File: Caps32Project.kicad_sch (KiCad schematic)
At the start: 35 parts, among them J1 PH2.0, J2 USB_C_Receptacle_USB2.0_16P, J3 SH1.0, Q1 AO3401A, SW1 Boot, SW2 Reset, SW3 SW_SPDT_312, U1 TP4057, U2 MPU-6050, U3 ESP32-C3-MINI-1, U4 AP2112K-3.3

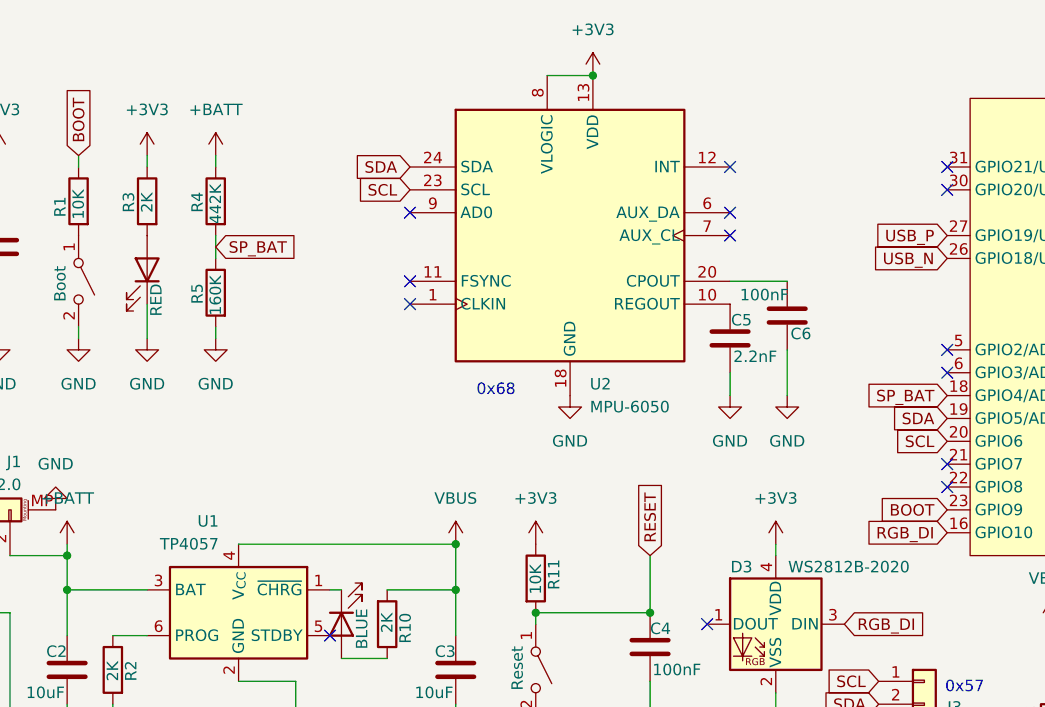
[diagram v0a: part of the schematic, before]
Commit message: Update Board
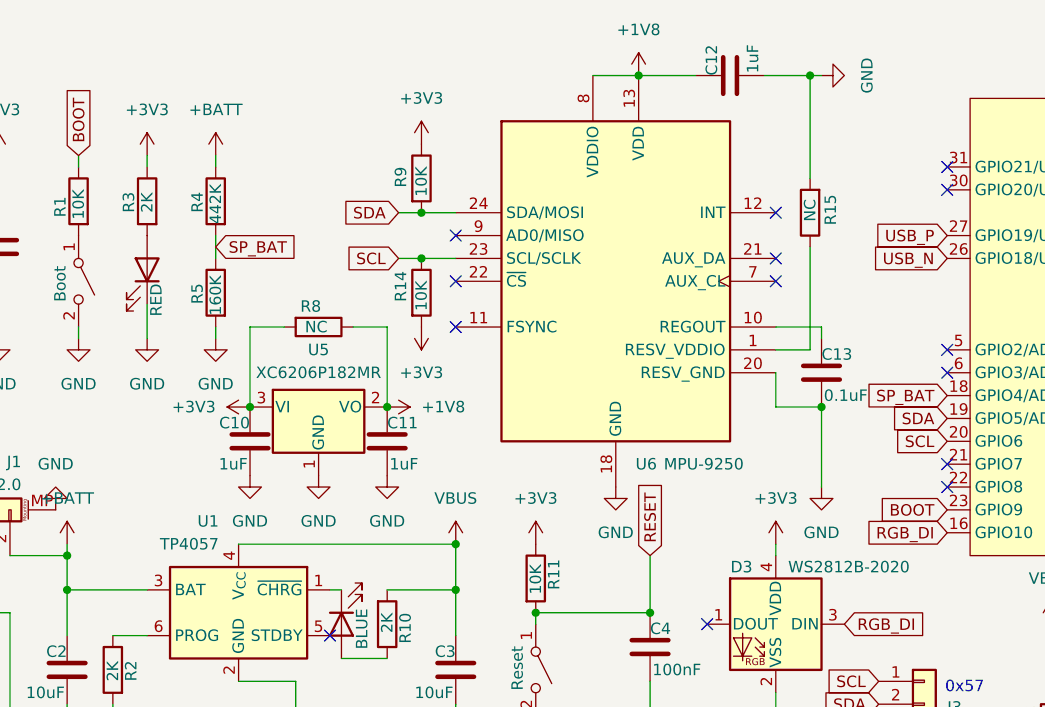
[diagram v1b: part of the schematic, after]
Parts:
- removed C5: 2.2nF, Capacitor_SMD:C_0603_1608Metric, symbol Device:C
- removed C6: 100nF, Capacitor_SMD:C_0402_1005Metric, symbol Device:C
- removed U2: MPU-6050, Sensor_Motion:InvenSense_QFN-24_4x4mm_P0.5mm, symbol Sensor_Motion:MPU-6050
- added C10, C11, C12: 1uF, Capacitor_SMD:C_0402_1005Metric, symbol Device:C
- added C13: 0.1uF, Capacitor_SMD:C_0402_1005Metric, symbol Device:C
- added R14, R9: 10K, Resistor_SMD:R_0402_1005Metric, symbol Device:R
- added R15, R8: NC, Resistor_SMD:R_0402_1005Metric, symbol Device:R
- added U5: XC6206P182MR, Package_TO_SOT_SMD:SOT-23-3, symbol Regulator_Linear:XC6206PxxxMR
- added U6: MPU-9250, Sensor_Motion:InvenSense_QFN-24_3x3mm_P0.4mm, symbol Sensor_Motion:MPU-9250
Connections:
- net +3V3: now also C10.1, R14.2, R8.2, R9.1, U5.3 (VI)
- net GND: now also C10.2, C11.2, C12.2, C13.2, R15.2, U5.1 (GND), U6.18 (GND), U6.20 (RESV_GND)
- net SCL: now also R14.1, U6.23 (SCL/SCLK)
- net SDA: now also R9.2, U6.24 (SDA/MOSI)
- new net: R15.1, U6.1 (RESV_VDDIO)
- new net: C13.1, U6.10 (REGOUT)
- new net +1V8: C11.1, C12.1, R8.1, U5.2 (VO), U6.13 (VDD), U6.8 (VDDIO)
